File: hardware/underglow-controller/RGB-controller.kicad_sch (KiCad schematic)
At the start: 0 parts

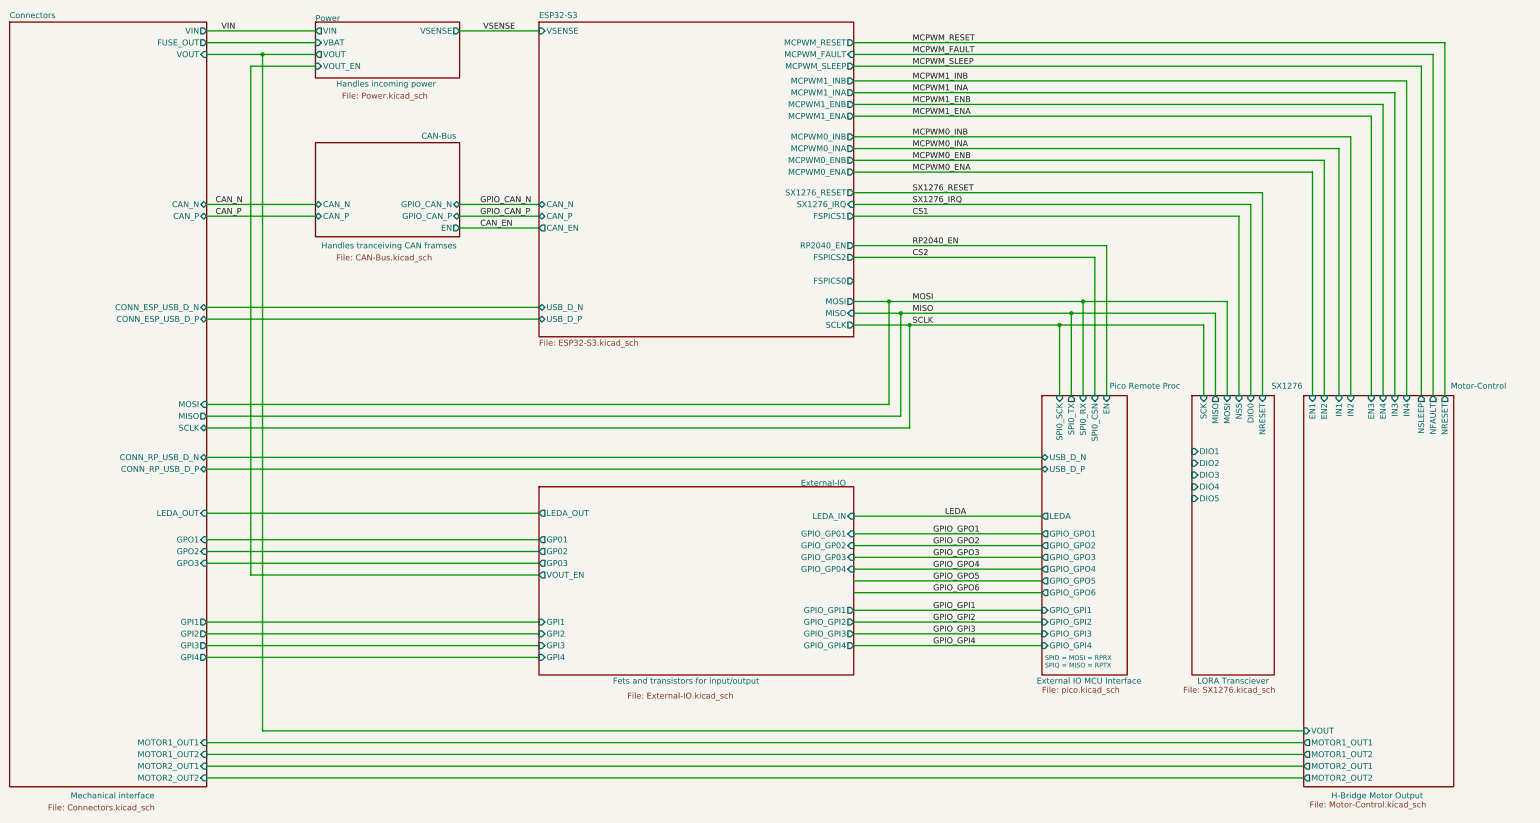
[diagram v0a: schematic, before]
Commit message: iasdf
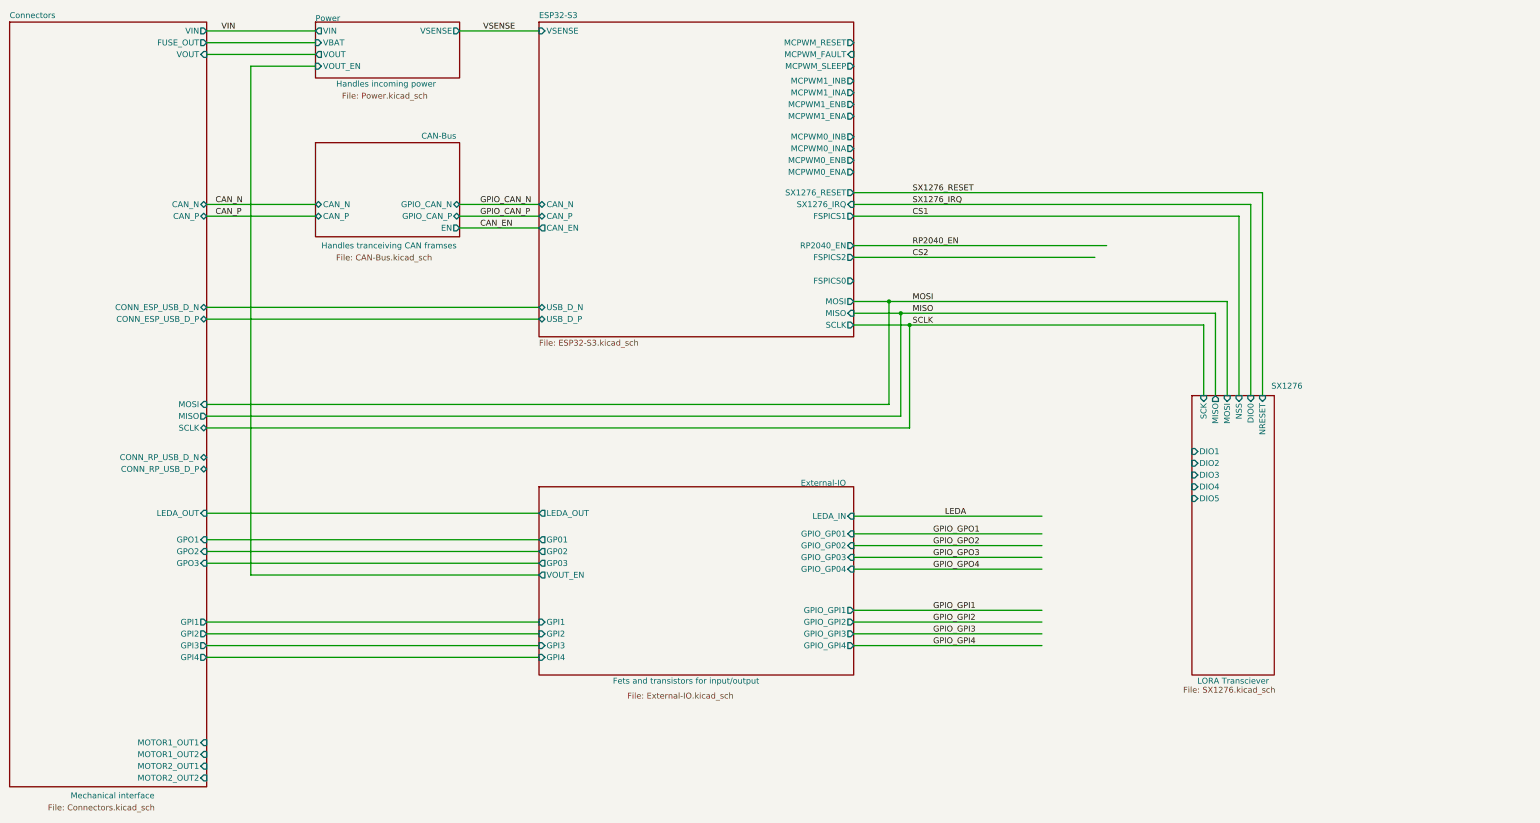
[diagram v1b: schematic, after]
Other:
- removed sheet Motor-Control
- removed sheet Pico Remote Proc
- note removed: "SPID = MOSI = RPRX SPIQ = MISO = RPTX"
